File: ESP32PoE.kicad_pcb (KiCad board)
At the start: 4 copper layers, 90 x 40 mm, 56 parts, among them J1 Conn_01x20_Pin, J2 Conn_01x20_Pin, J3 Conn_01x04_Pin, SW1 SW_Push, SW2 SW_Push, U1 W5500, U2 MagJack-A70-112-331N126, U3 AMS1117-3.3, U4 ESP32-S3-WROOM-1, U7 AG9905LP, Y1 XO32F025000GEHE001

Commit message: fix: board notes
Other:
- board text added: "0.0152 mm"
- board text added: "0.15 mm / 0.127 mm"
- board text added: "0.2104 mm"
- board text added: "1.065 mm"
- board text added: "1.6062 mm"
- board text removed: "0.03 mm"
- board text removed: "0.2 mm / 0.2 mm"
- board text removed: "0.203 mm"
- board text removed: "1.03 mm"
- board text removed: "1.586 mm"
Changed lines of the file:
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@@
 		)
 	)
-	(gr_text "0.203 mm"
+	(gr_text "0.2104 mm"
 		(at 87.342857 160.845 0)
 		(layer "Cmts.User")
@@
 		)
 	)
-	(gr_text "0.203 mm"
+	(gr_text "0.2104 mm"
 		(at 87.342857 143.985 0)
 		(layer "Cmts.User")
@@
 		)
 	)
-	(gr_text "0.03 mm"
+	(gr_text "0.0152 mm"
 		(at 87.342857 148.2 0)
 		(layer "Cmts.User")
@@
 		)
 	)
-	(gr_text "1.586 mm"
+	(gr_text "1.6062 mm"
 		(at 261.3 128.54 0)
 		(layer "Cmts.User")
@@
 		)
 	)
-	(gr_text "0.2 mm / 0.2 mm"
+	(gr_text "0.15 mm / 0.127 mm"
 		(at 199.542857 137.57 0)
 		(layer "Cmts.User")
@@
 		)
 	)
-	(gr_text "1.03 mm"
+	(gr_text "1.065 mm"
 		(at 87.342857 152.415 0)
 		(layer "Cmts.User")
@@
 		)
 	)
-	(gr_text "0.03 mm"
+	(gr_text "0.0152 mm"
 		(at 87.342857 156.63 0)
 		(layer "Cmts.User")

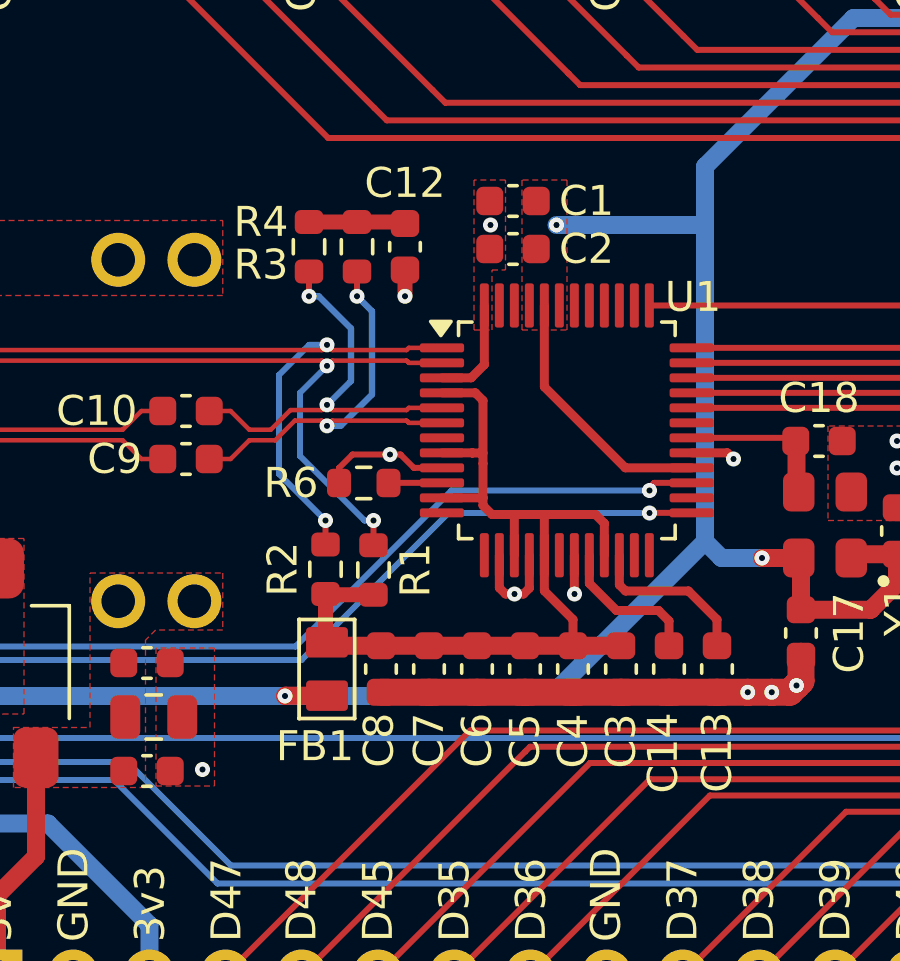
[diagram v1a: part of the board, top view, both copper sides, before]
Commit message: wip: minor adjustments
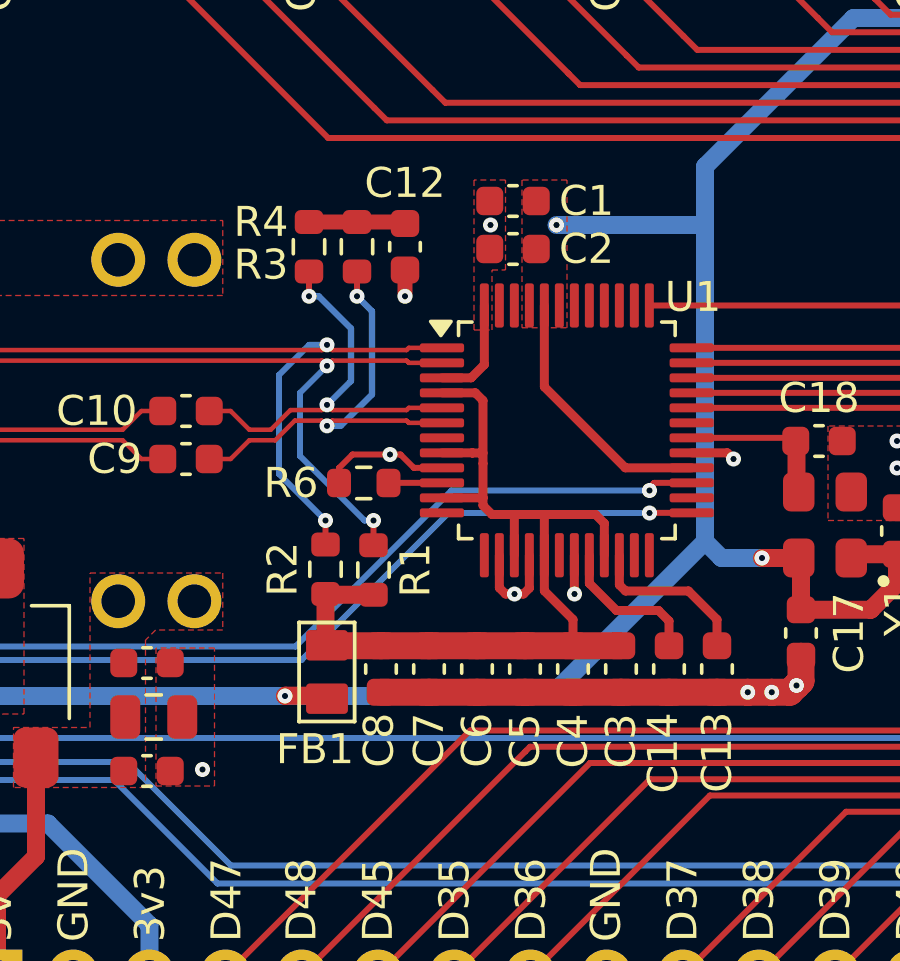
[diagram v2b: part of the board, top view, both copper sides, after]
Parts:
- moved FB1 0.10 mm to (139.2, 88.1)
